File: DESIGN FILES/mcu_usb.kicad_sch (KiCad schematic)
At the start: 26 parts, among them J401 YTC-TC16S-28, Q401 MMBT3904, Q402 MMBT3904, SW401 TS-1187A-B-A-B, U401 ESP32-WROVER-E-N4R8, U402 CP2102N-A02-GQFN28R

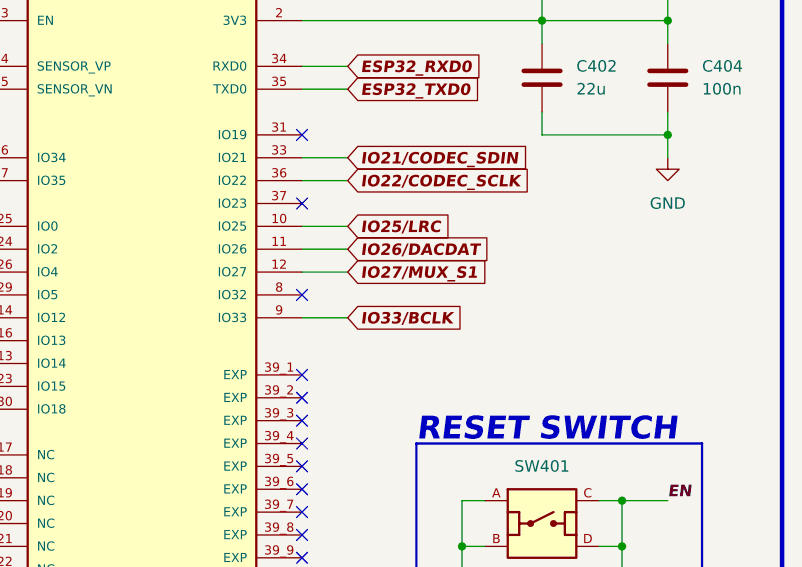
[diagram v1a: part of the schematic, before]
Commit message: updates
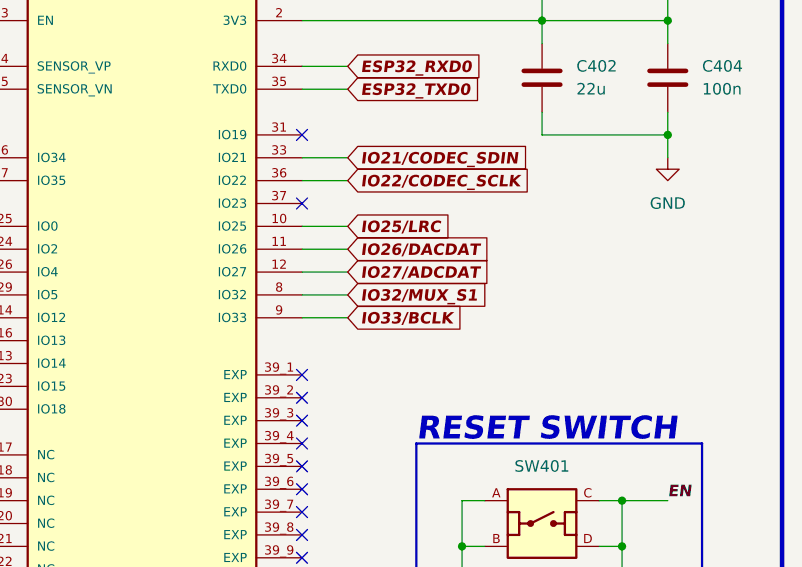
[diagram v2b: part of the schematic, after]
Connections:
- net IO32/MUX_S1: now reaches U401.8 (IO32)
- net IO27/MUX_S1 renamed IO27/ADCDAT
- no-connect marks 35 -> 34
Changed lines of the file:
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@@
   (no_connect (at 339.09 135.89))
   (no_connect (at 339.09 120.65))
-  (no_connect (at 339.09 106.68))
   (no_connect (at 339.09 88.9))
   (no_connect (at 339.09 96.52))
@@
     (stroke (width 0) (type default) (color 0 0 0 0))
   )
+  (wire (pts (xy 339.09 106.68) (xy 344.17 106.68))
+    (stroke (width 0) (type default) (color 0 0 0 0))
+  )
   (polyline (pts (xy 392.43 63.5) (xy 392.43 158.75))
     (stroke (width 0.5) (type default) (color 0 0 0 0))
@@
     )
   )
+  (global_label "IO32{slash}MUX_S1" (shape input) (at 344.17 106.68 0) (fields_autoplaced)
+    (effects (font (size 1.27 1.27) (thickness 0.254) bold italic) (justify left))
+    (property "Intersheet References" "${INTERSHEET_REFS}" (id 0) (at 360.0919 106.553 0)
+      (effects (font (size 1.27 1.27) (thickness 0.254) bold italic) (justify left) hide)
+    )
+  )
   (global_label "IO0{slash}MCLK" (shape input) (at 297.18 99.06 180) (fields_autoplaced)
     (effects (font (size 1.27 1.27) (thickness 0.254) bold italic) (justify right))
@@
     )
   )
-  (global_label "IO27{slash}MUX_S1" (shape input) (at 344.17 104.14 0) (fields_autoplaced)
+  (global_label "IO27{slash}ADCDAT" (shape input) (at 344.17 104.14 0) (fields_autoplaced)
     (effects (font (size 1.27 1.27) (thickness 0.254) bold italic) (justify left))
-    (property "Intersheet References" "${INTERSHEET_REFS}" (id 0) (at 360.0919 104.013 0)
+    (property "Intersheet References" "${INTERSHEET_REFS}" (id 0) (at 359.6686 104.013 0)
       (effects (font (size 1.27 1.27) (thickness 0.254) bold italic) (justify left) hide)
     )

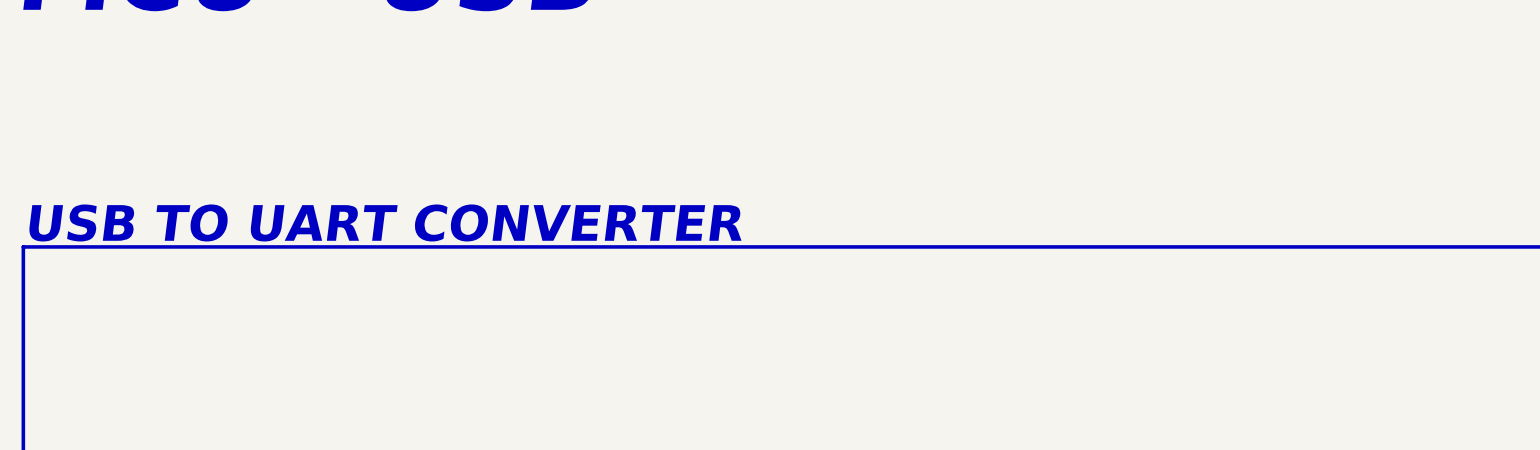
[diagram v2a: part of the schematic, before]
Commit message: updates
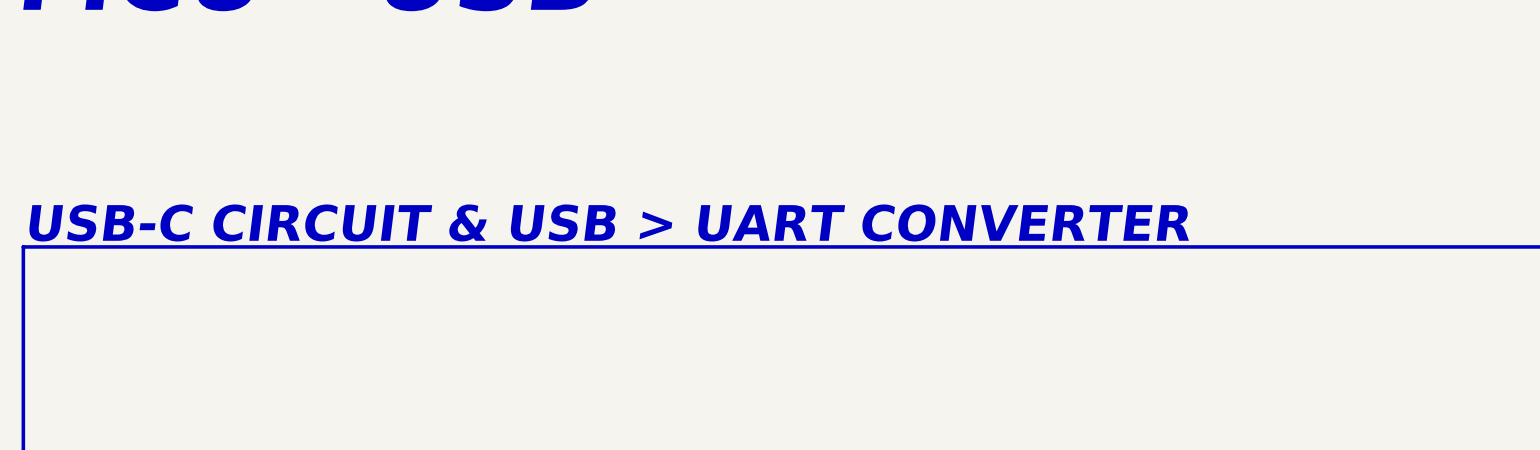
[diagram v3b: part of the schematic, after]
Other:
- note added: "USB-C CIRCUIT & USB > UART CONVERTER"
- note removed: "USB TO UART CONVERTER"
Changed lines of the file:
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@@
     (stroke (width 0) (type default) (color 0 0 0 0))
   )
-  (text "USB TO UART CONVERTER" (at 26.67 63.5 0)
+  (text "USB-C CIRCUIT & USB > UART CONVERTER" (at 26.67 63.5 0)
     (effects (font (size 5 5) bold italic) (justify left bottom))
   )
